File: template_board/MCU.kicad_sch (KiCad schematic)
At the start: 33 parts, among them J3 SWD, SW6 NRST, U5 STM32U575RITx, X3 Q13FC1350000400, X4 X322512MSB4SI

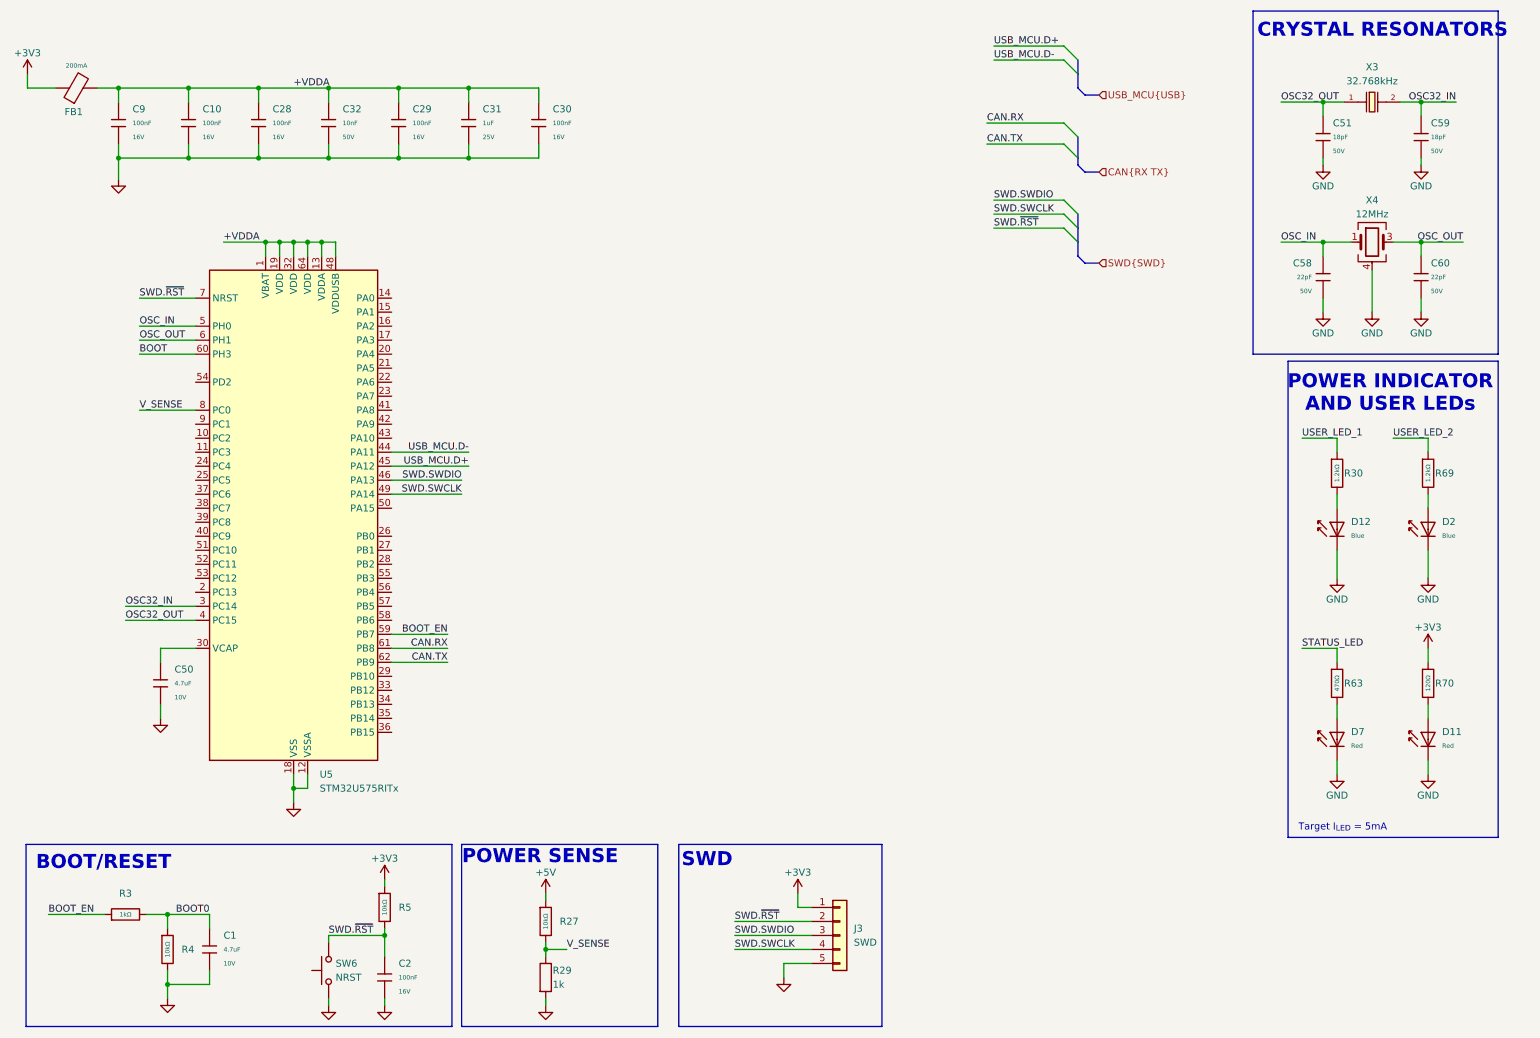
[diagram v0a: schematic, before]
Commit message: chamt skończony chyba
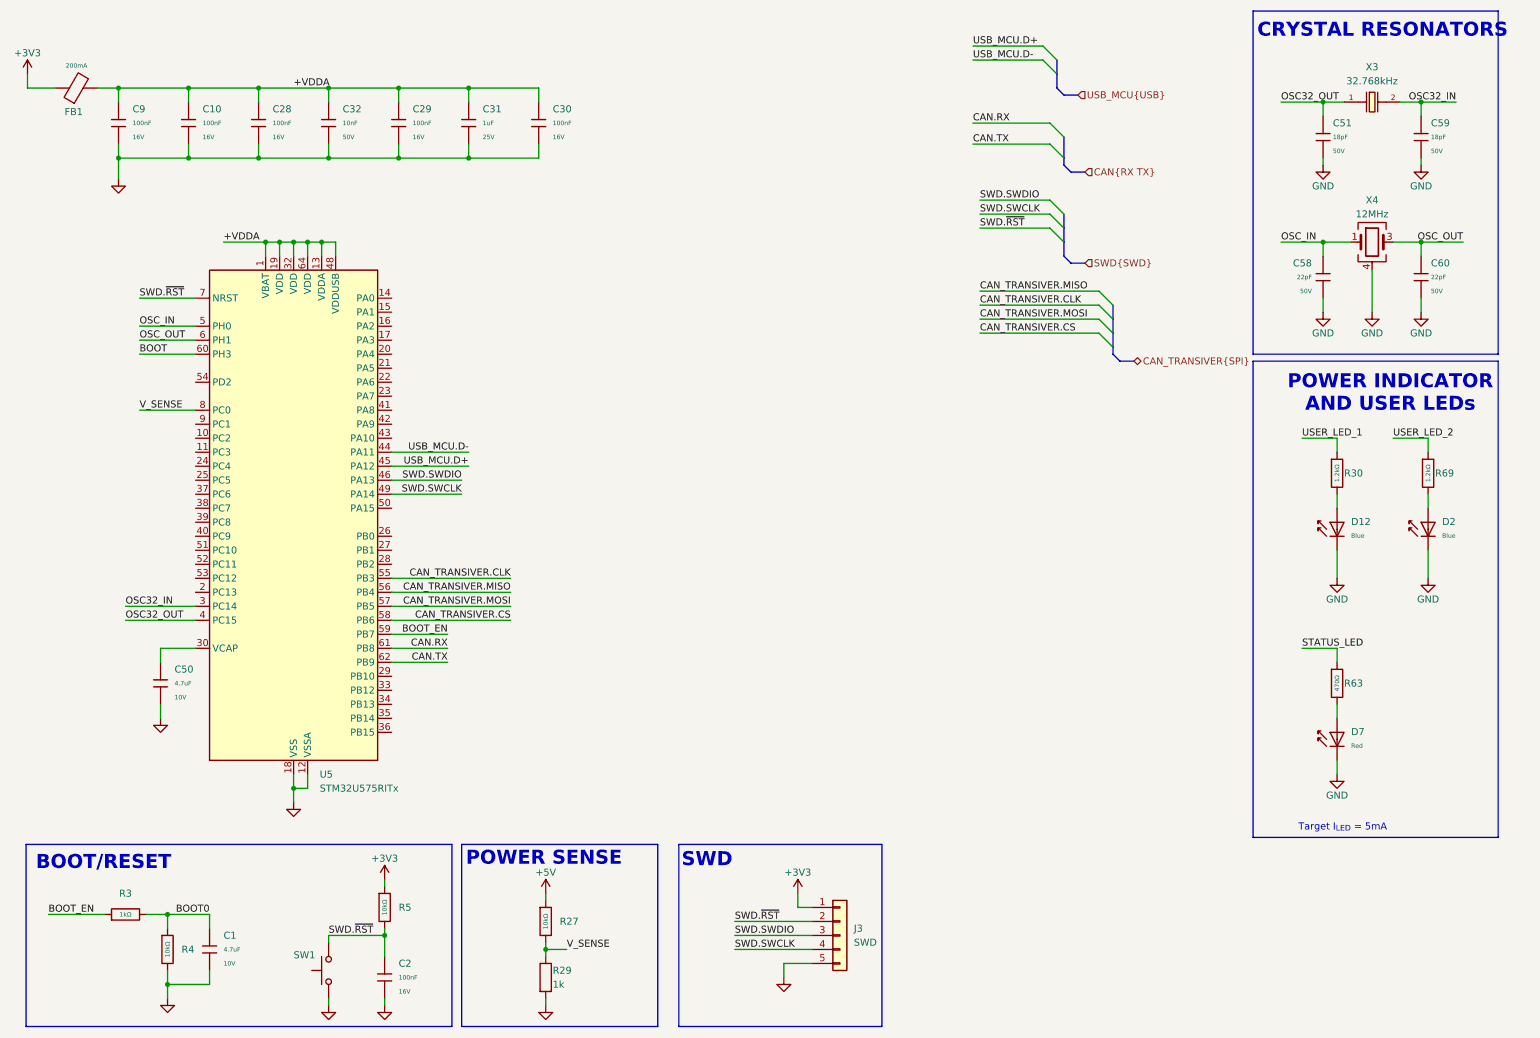
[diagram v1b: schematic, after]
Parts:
- removed D11: Red, PCM_JLCPCB:D_0603, symbol PCM_JLCPCB-Diodes:LED,0603,Red
- removed R70: 120Ω, PCM_JLCPCB:R_0402, symbol PCM_JLCPCB-Resistors:0402,120Ω
- removed SW6: NRST, Button_Switch_THT:SW_Tactile_SPST_Angled_PTS645Vx58-2LFS, symbol Switch:SW_Push
- added SW1: SW_Push, lib:TS1088R02026, symbol Switch:SW_Push
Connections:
- net GND: now also SW1.1
- net SWD.~{RST}: now also SW1.2
- net CAN_TRANSIVER.CLK: now reaches U5.55 (PB3)
- net CAN_TRANSIVER.MISO: now reaches U5.56 (PB4)
- net CAN_TRANSIVER.MOSI: now reaches U5.57 (PB5)
- net CAN_TRANSIVER.CS: now reaches U5.58 (PB6)
